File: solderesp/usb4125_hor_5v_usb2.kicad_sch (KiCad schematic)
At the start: 14 parts, among them J3 USB4105-GF-A

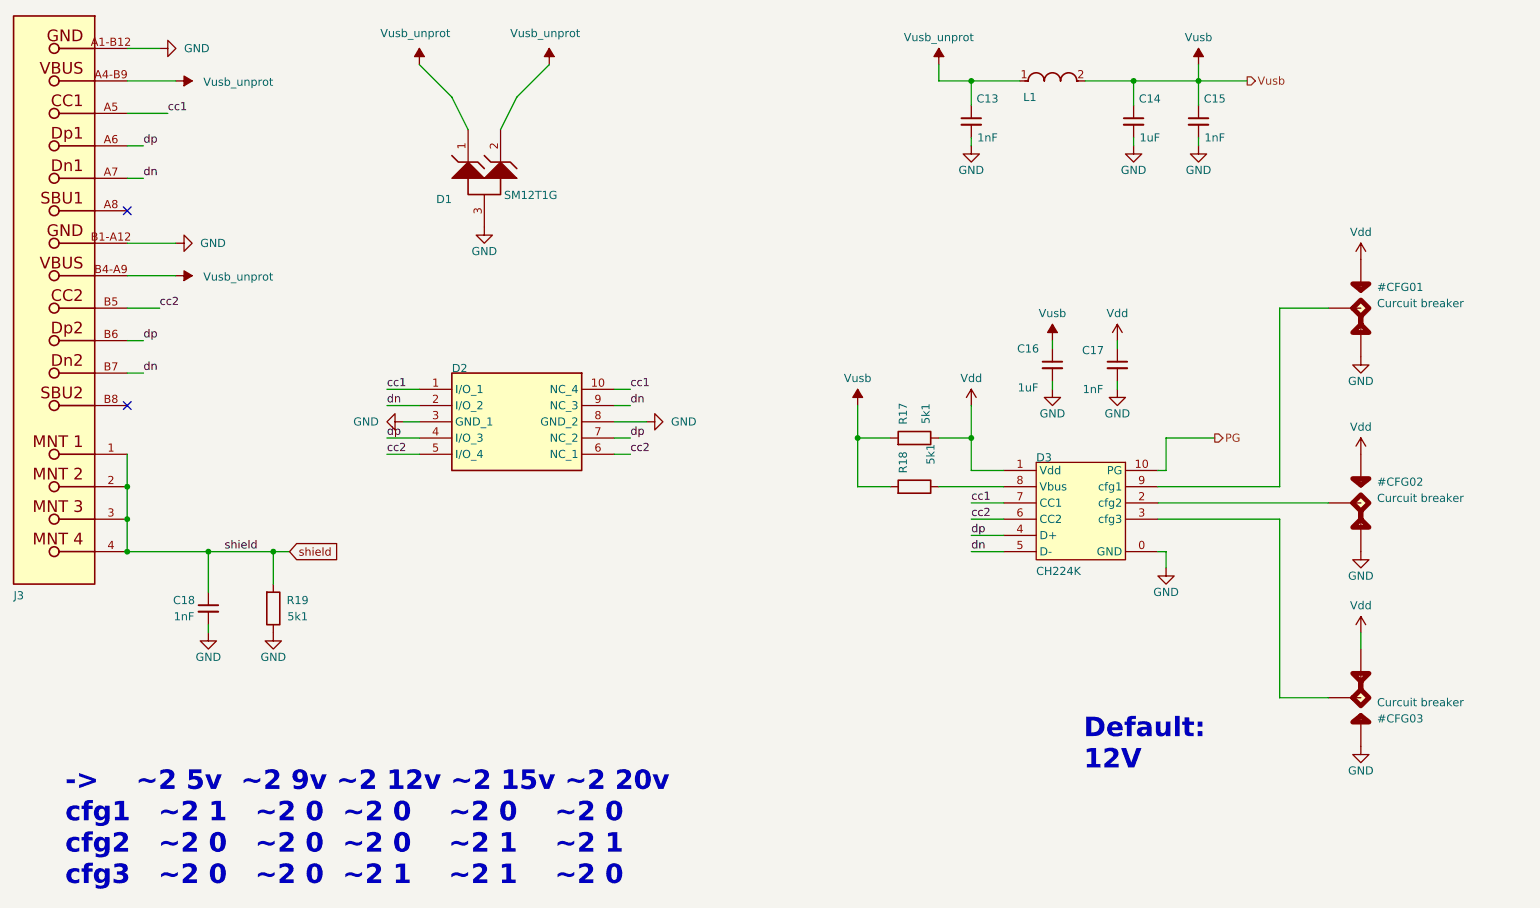
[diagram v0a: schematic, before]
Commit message: Required symbols SCH & 3D has been added
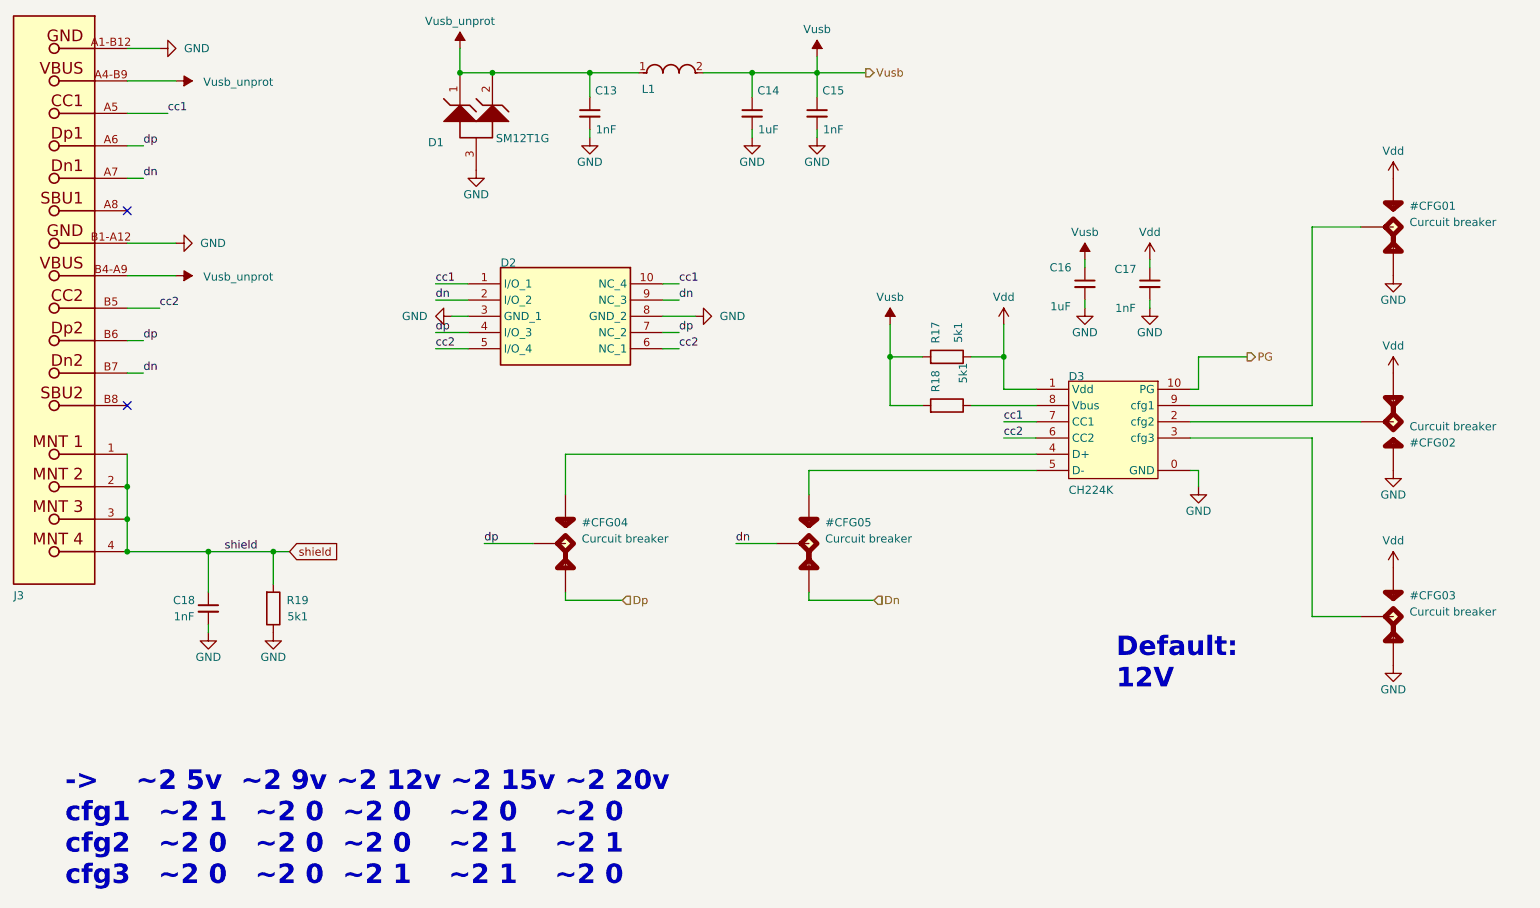
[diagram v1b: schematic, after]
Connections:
- net dn: no longer D3.5 (D-)
- net dp: no longer D3.4 (D+)
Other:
- moved on the sheet: C13, C14, C15, C16, C17, D1, D2, D3, L1, R17, R18
